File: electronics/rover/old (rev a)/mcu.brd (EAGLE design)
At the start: 46.3 x 25.4 mm, 34 parts, among them IC1 24LC128SM, IC2 24LC128SM, J1 AVR_SPI_PRG_62X3_LOCK, M1 M02PTH, M2 M02PTH, Q2 16M, U1 DRV8833_PWP_16, U2 MPL3115A2LGA8, U4 ATMEGA328P

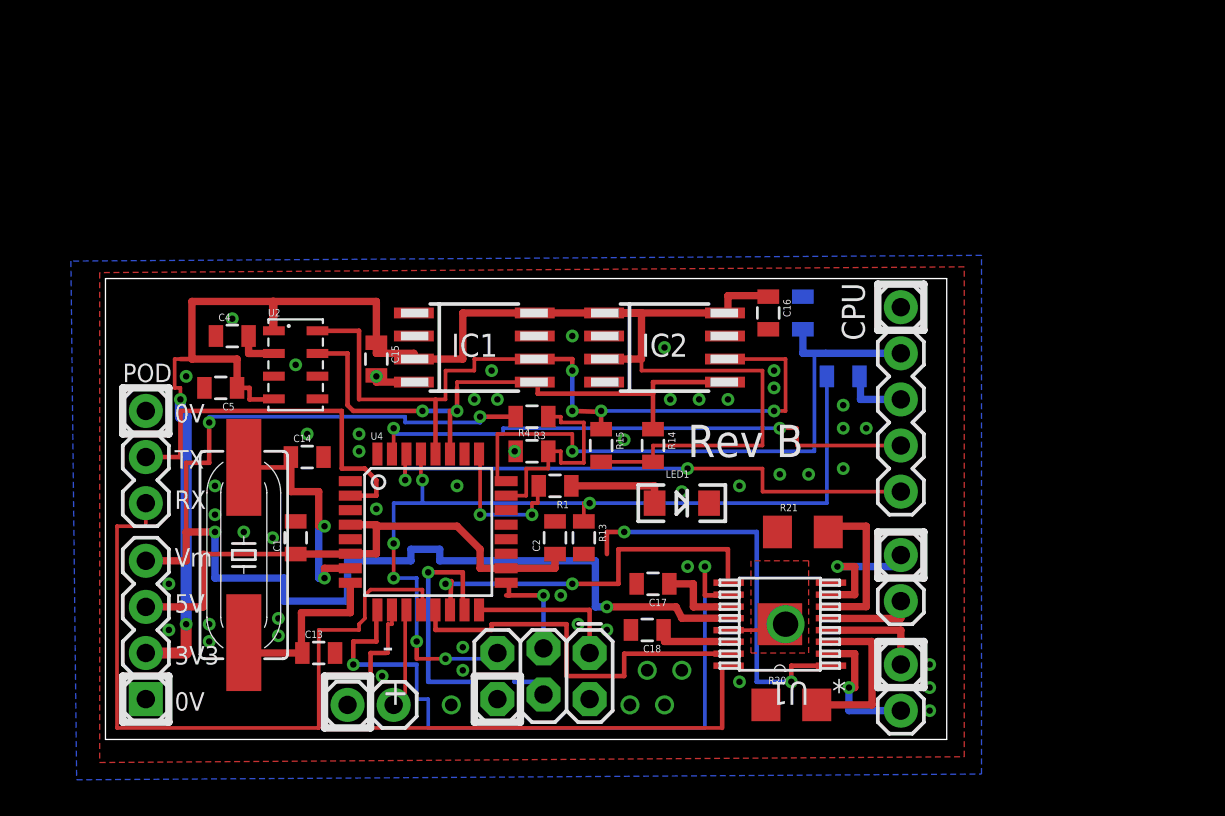
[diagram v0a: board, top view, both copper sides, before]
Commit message: Added new electronic designs
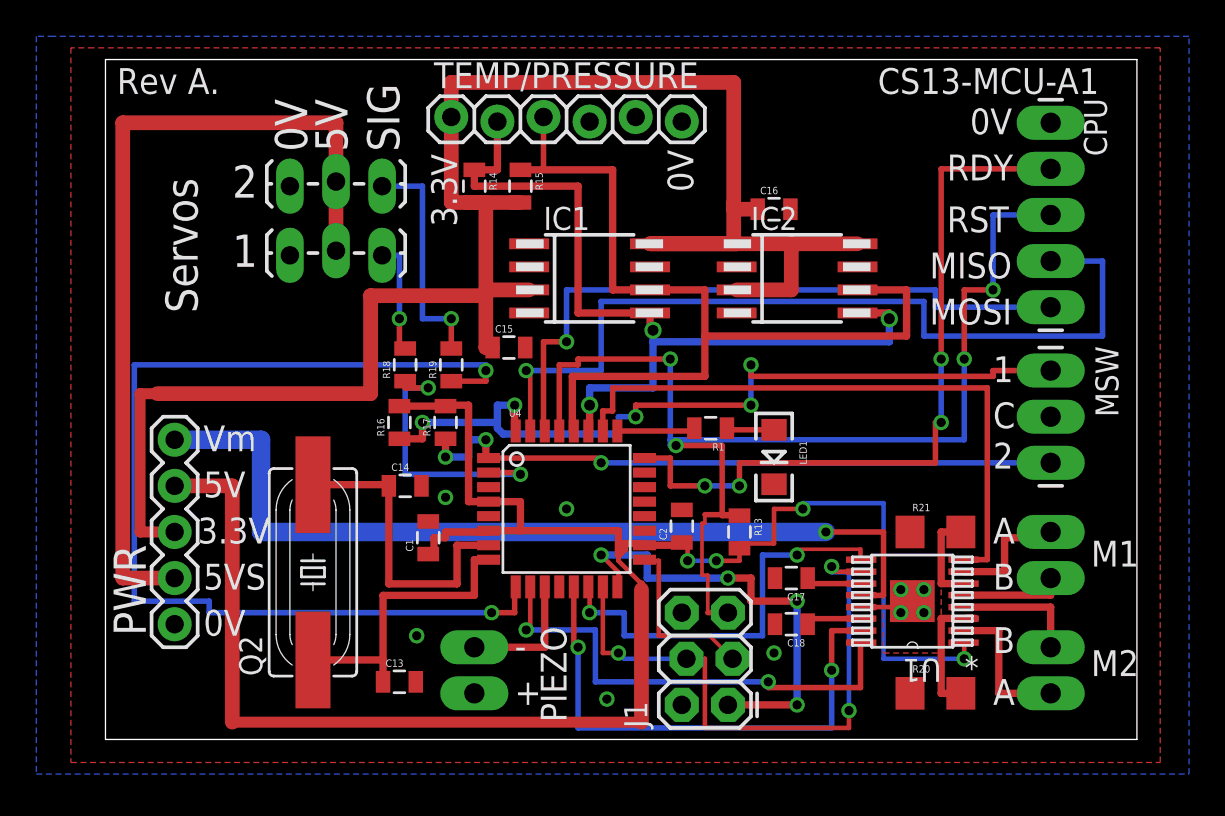
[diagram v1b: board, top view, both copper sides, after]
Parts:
- removed C3, C4: 100nF, SparkFun-Capacitors:0805
- removed C5: 1u, SparkFun-Passives:0805
- removed POD: (no value), SparkFun-Connectors:1X03
- removed R2: 4.7k, SparkFun-Passives:0805
- removed R3: 22k, SparkFun-Passives:0805
- removed R4: 10k, SparkFun-Passives:0805
- removed U2: MPL3115A2LGA8, SparkFun-Sensors:LGA8
- added JP3: (no value), SparkFun-Connectors:1X03_LOCK_LONGPADS
- added MCU_PWR: (no value), SparkFun-Connectors:1X05
- added MSW: (no value), SparkFun-Connectors:1X03_LONGPADS
- added R16, R17: 10k, SparkFun-Passives:0805
- added R18, R19: 100, SparkFun-Passives:0805
- added TPS: (no value), SparkFun-Connectors:1X06_LOCK
- CPU: device SparkFun-Connectors:1X05 -> SparkFun-Connectors:1X05_LONGPADS
- JP1, M1, M2: value M02PTH -> (none); device SparkFun-Connectors:1X02 -> SparkFun-Connectors:1X02_LONGPADS
- JP2: device SparkFun-Connectors:1X04 -> SparkFun-Connectors:1X03_LOCK_LONGPADS
- moved JP2 27.7 mm to (15.2, 26.7), turned to 180 degrees
- moved R14 17.3 mm to (20.3, 30.5)
- moved R15 15.0 mm to (22.9, 30.5)
- moved CPU 13.1 mm to (52.1, 34.0)
- moved R1 9.14 mm to (33.3, 17.1)
- moved R13 8.58 mm to (34.9, 11.4)
- moved M2 8.35 mm to (52.1, 11.4)
- moved M1 8.31 mm to (52.1, 2.54)
- moved IC2 8.24 mm to (38.1, 25.4)
- moved J1 8.14 mm to (34.3, 1.91), turned to 90 degrees
- moved R20 7.96 mm to (45.7, 2.54)
- moved C18 7.94 mm to (37.8, 6.35)
- moved U4 7.73 mm to (25.4, 12.7)
- moved C17 7.63 mm to (37.8, 8.89)
- moved U1 7.41 mm to (44.5, 7.62)
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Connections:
- net AIS renamed N$25
- net BIS renamed N$24
- net ISP_MISO renamed N$19
- net ISP_SCK renamed N$18
- net STAT_LED renamed N$1
- net VCP renamed N$21
- net VINT renamed N$23
- removed net CAP: C4.2, U2.2
- removed net ISP_MOSI: J1.4, U4.15
- removed net LNK_RST: C3.1, CPU.3
- removed net MON: R3.1, R4.2, U4.23
- removed net POD_MISO: POD.2, U4.2
- removed net POD_MOSI: POD.1, U4.12
- new net 5VS: JP2.2, JP3.2, MCU_PWR.2
- new net FLT: U1.8, U4.26
- new net N$17: JP2.1, R18.2
- new net N$20: JP3.1, R19.2
- new net SERVO1: R18.1, U4.2
- new net SERVO2: R19.1, U4.9
- new net SW1: MSW.1, R16.1, U4.32
- new net SW2: MSW.3, R17.1, U4.1
- net 3.3V: now also MCU_PWR.3, TPS.1; no longer C5.1, JP2.2, U2.1, U2.4
- net 5V: now also MCU_PWR.4, R16.2, R17.2; no longer JP2.3
- net GND: now also JP2.3, JP3.3, MCU_PWR.1, MSW.2, TPS.6; no longer C4.1, C5.2, JP2.1, POD.3, R2.1, R4.1, U2.3
- net M2B_CTL: now also J1.4, U4.15; no longer U4.9
- net RDY: no longer R2.2
- net RST: now also CPU.3; no longer C3.2
- net SCL: now also TPS.3; no longer U2.8
- net SDA: now also TPS.2; no longer U2.7
- net V_BATT: now also MCU_PWR.5; no longer JP2.4, R3.2
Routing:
- net SERVO2: track 0.00 -> 58.3 mm, vias 0 -> 2
- net 5V: track 53.6 -> 108.6 mm, vias 2 -> 4
- net 5VS: track 0.00 -> 46.7 mm
- net SW1: track 0.00 -> 45.4 mm, vias 0 -> 5
- net POD_MOSI: track 39.2 -> 0.00 mm
- net SW2: track 0.00 -> 36.6 mm, vias 0 -> 3
- net FLT: track 0.00 -> 34.3 mm
- net POD_MISO: track 21.0 -> 0.00 mm
- net V_BATT: track 69.1 -> 48.9 mm, vias 4 -> 1
- net ISP_MOSI: track 17.7 -> 0.00 mm, vias 1 -> 0
- net LNK_MISO: track 31.0 -> 48.1 mm, vias 2 -> 1
- net N$19: track 8.46 -> 25.1 mm, vias 0 -> 4
- net SERVO1: track 0.00 -> 15.9 mm, vias 0 -> 2
- net RST: track 49.6 -> 64.7 mm, vias 6 -> 4
- net SDA: track 33.0 -> 48.1 mm, vias 2 -> 3
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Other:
- board size 46.3 x 25.4 mm -> 56.8 x 37.5 mm
- board text added: "1"
- board text added: "2"
- board text added: "3.3V"
- board text added: "5VS"
- board text added: "A"
- board text added: "B"
- board text added: "C"
- board text added: "CS13-MCU-A1"
- board text added: "CanSat MCU Board"
- board text added: "M1"
- board text added: "M2"
- board text added: "MISO"
- board text added: "MOSI"
- board text added: "PIEZO"
- board text added: "PWR"
- board text added: "RDY"
- board text added: "RST"
- board text added: "Rev A."
- board text added: "SIG"
- board text added: "Servos"
- board text added: "TEMP/PRESSURE"
- board text removed: "3V3"
- board text removed: "CS13-MCU-B1"
- board text removed: "POD"
- board text removed: "RX"
- board text removed: "Rev B"
- board text removed: "TX"
